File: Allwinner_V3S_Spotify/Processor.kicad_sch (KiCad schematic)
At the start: 1 part

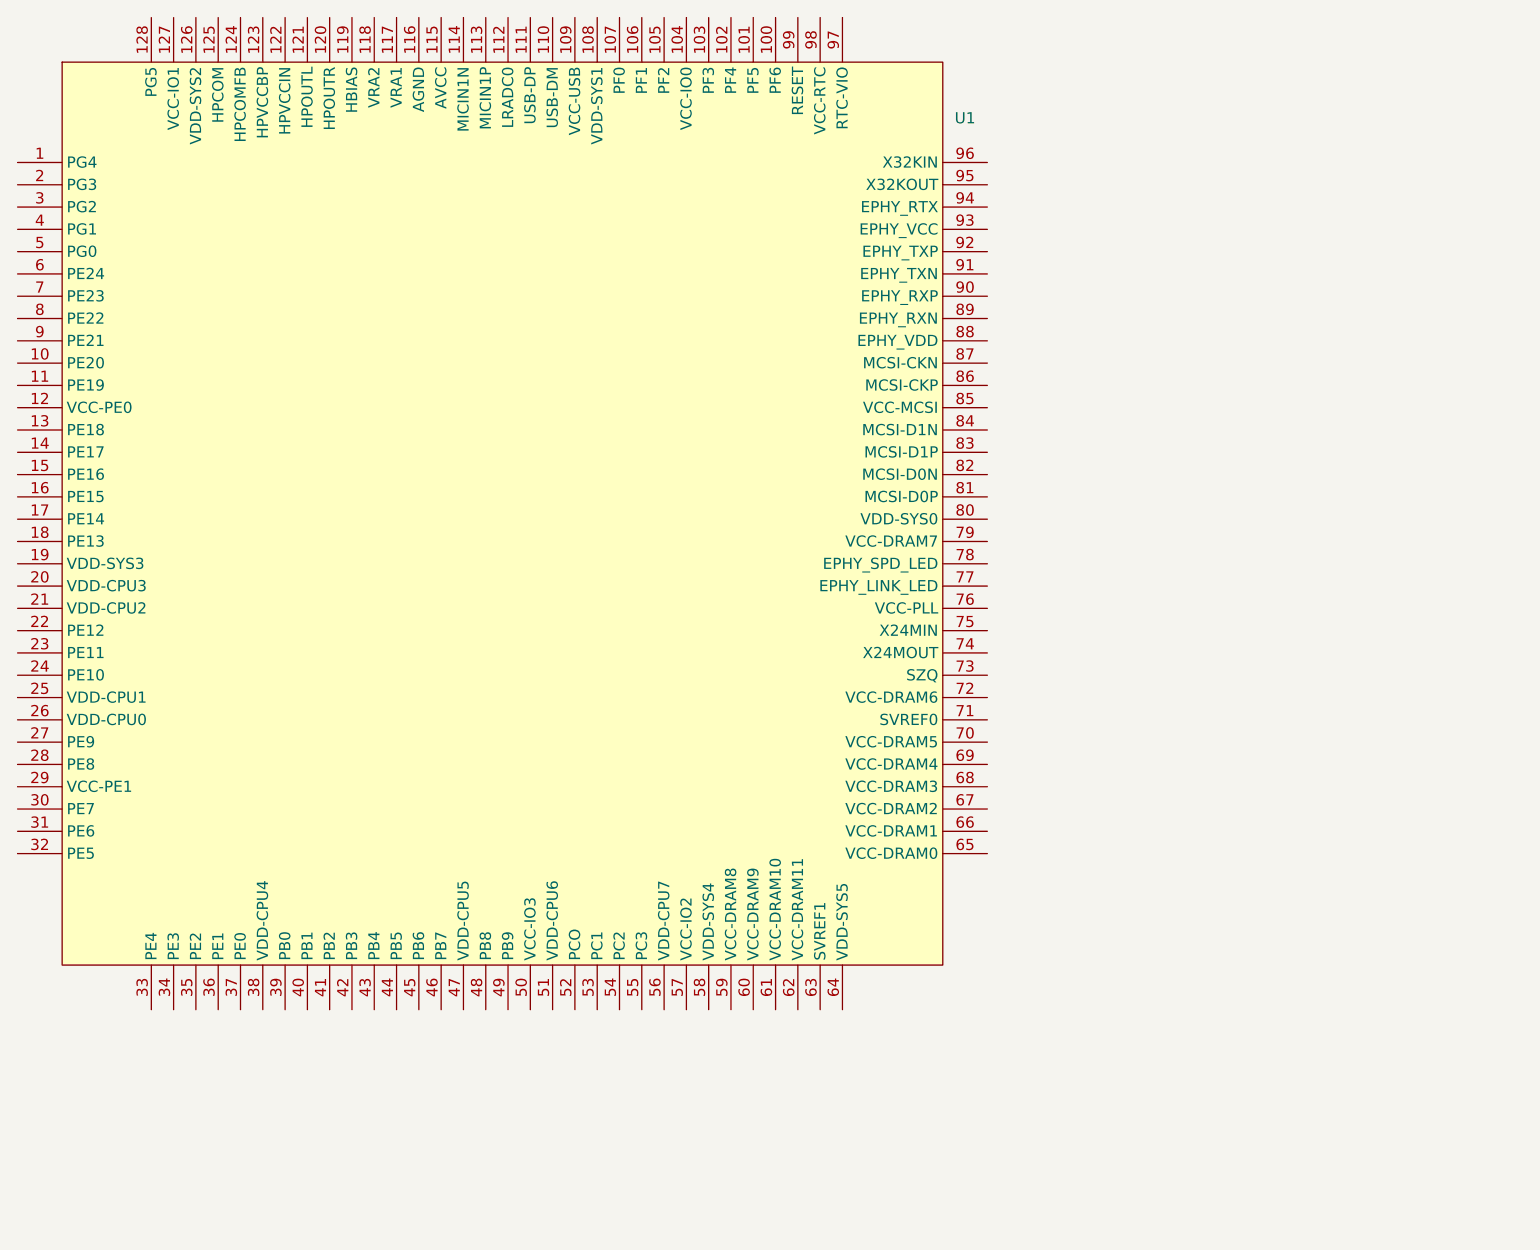
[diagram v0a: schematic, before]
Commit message: More work on Schematics
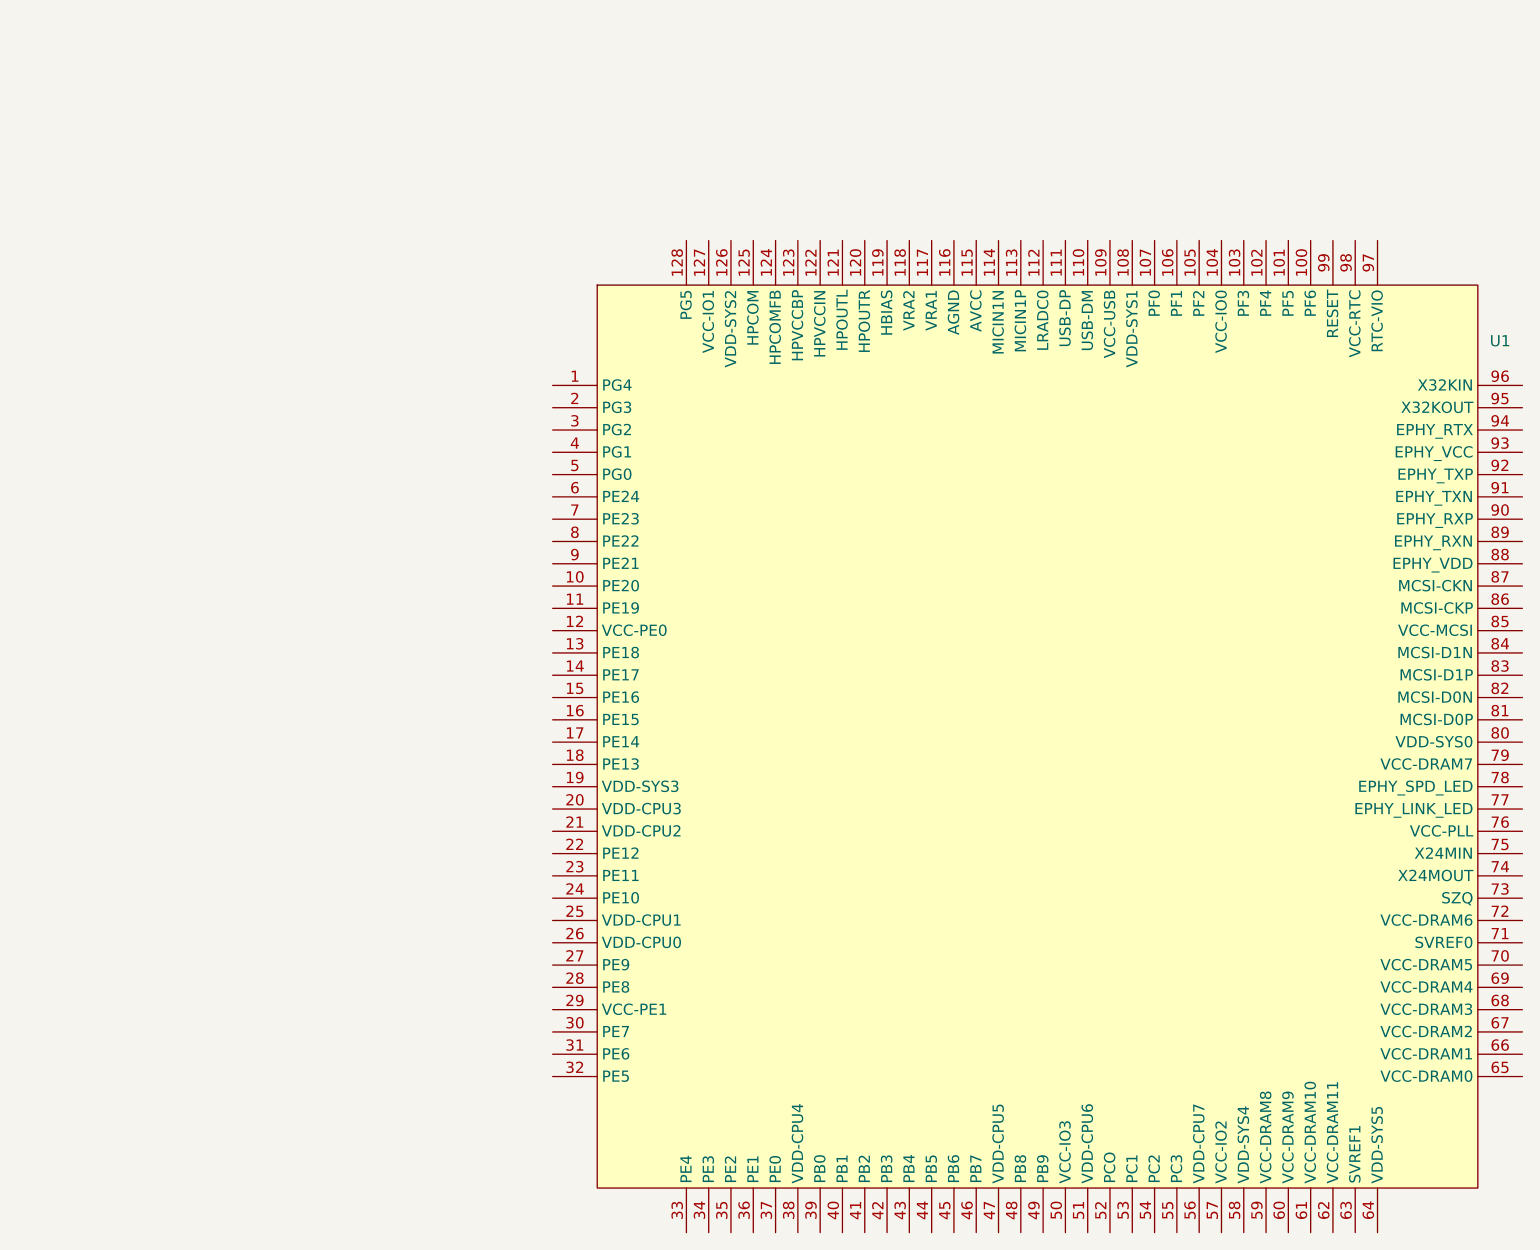
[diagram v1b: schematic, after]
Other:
- moved on the sheet: U1
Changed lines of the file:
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@@
 	(generator "eeschema")
 	(generator_version "8.0")
-	(paper "A4")
+	(paper "A3")
 	(symbol
 		(lib_id "Allwinner_V3S_Spotify:ALLWINNER_V3S")
-		(at 144.78 90.17 0)
+		(at 205.74 115.57 0)
 		(unit 1)
 		(exclude_from_sim no)
@@
 		(fields_autoplaced yes)
 		(property "Reference" "U1"
-			(at 199.39 47.0214 0)
+			(at 260.35 72.4214 0)
 			(effects
 				(font
@@
 		)
 		(property "Value" "~"
-			(at 199.39 48.9265 0)
+			(at 260.35 74.3265 0)
 			(effects
 				(font
@@
 		)
 		(property "Footprint" "Allwinner_Spotify:LQFP-128_14x14mm_P0.4mm_EP"
-			(at 144.78 90.17 0)
+			(at 205.74 115.57 0)
 			(effects
 				(font
@@
 		)
 		(property "Datasheet" "https://linux-sunxi.org/images/2/23/Allwinner_V3s_Datasheet_V1.0.pdf"
-			(at 144.78 90.17 0)
+			(at 205.74 115.57 0)
 			(effects
 				(font
@@
 		)
 		(property "Description" "ARM Cortex-A7 CPU 1.2Ghz 512Mbit DDR2"
-			(at 144.78 90.17 0)
+			(at 205.74 115.57 0)
 			(effects
 				(font
@@
 		)
 		(property "OC_LCSC" "C2687449"
-			(at 144.78 90.17 0)
+			(at 205.74 115.57 0)
 			(effects
 				(font
